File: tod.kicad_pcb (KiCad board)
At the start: 2 copper layers, 72 x 57 mm, 67 parts, among them J1 Conn_01x04, J2 Conn_01x03, J3 Conn_01x04, J4 Conn_01x03, Q1 BC856B, Q2 BC817, Q3 BC856B, Q4 BC817, Q5 BC856, Q6 BC817, Q7 BC856, Q8 BC817, U1 PC817, U2 PC817, U3 PC817, U4 PC817

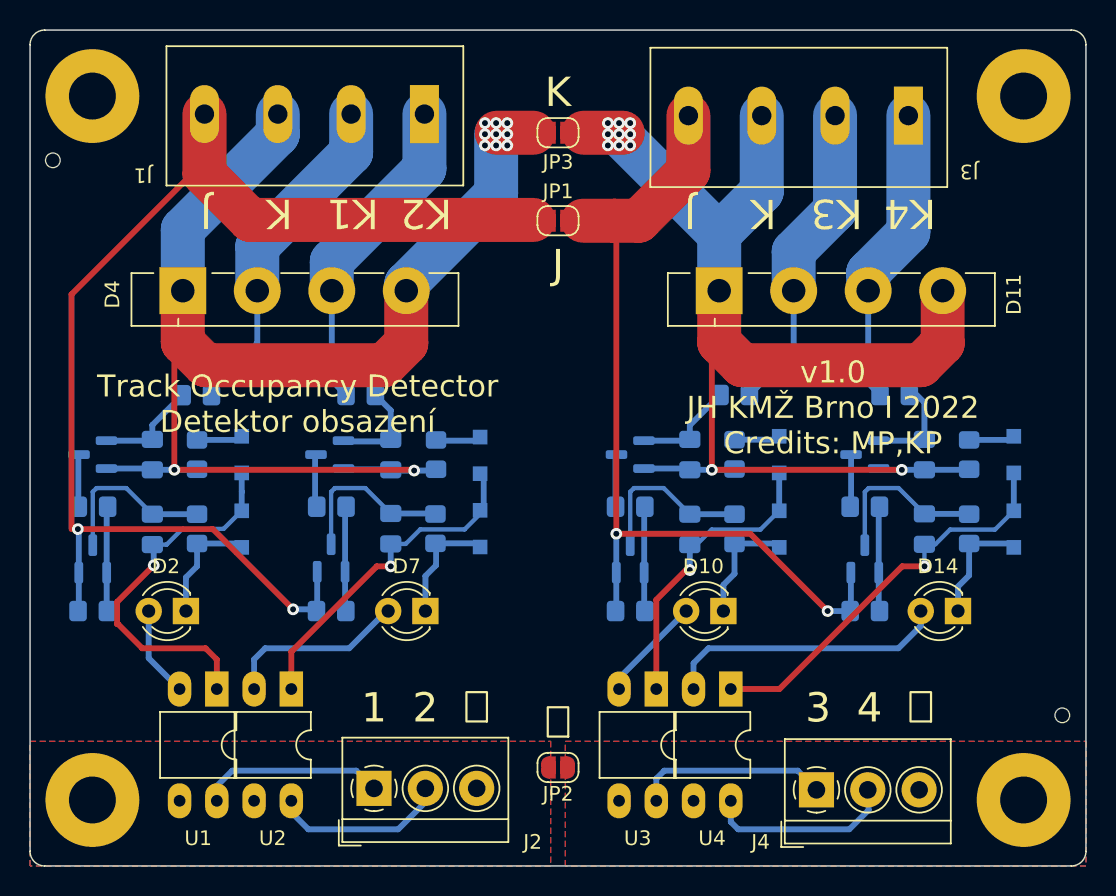
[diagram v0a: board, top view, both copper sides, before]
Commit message: Minor silkscreen tweaks.
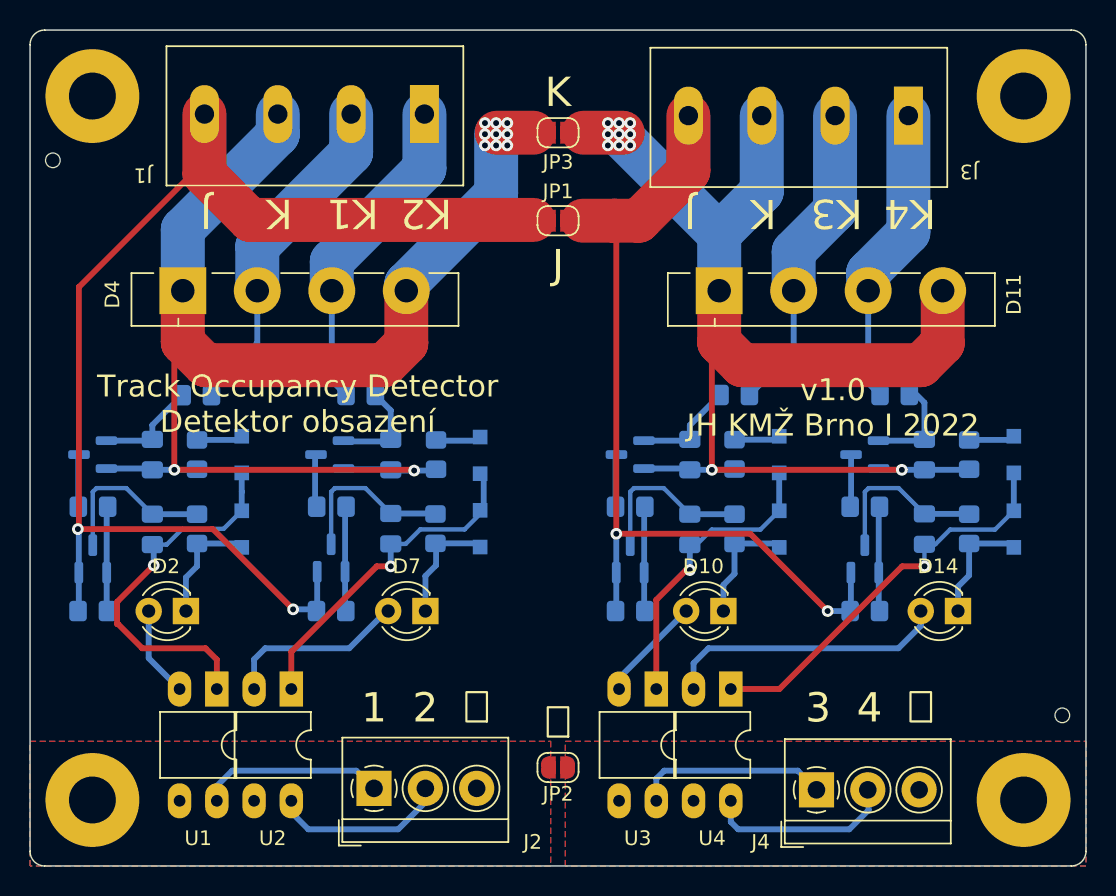
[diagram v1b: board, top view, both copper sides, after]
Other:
- board text added: "v1.0 JH KMŽ Brno I 2022"
- board text removed: "v1.0 JH KMŽ Brno I 2022 Credits: MP,KP"
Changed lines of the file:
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@@
     (effects (font (size 2 2) (thickness 0.15)))
   )
-  (gr_text "v1.0\nJH KMŽ Brno I 2022\nCredits: MP,KP" (at 167.75 88.75) (layer "F.SilkS")
+  (gr_text "v1.0\nJH KMŽ Brno I 2022" (at 167.75 88.75) (layer "F.SilkS")
     (effects (font (size 1.5 1.5) (thickness 0.15)))
   )
@@
   (segment (start 172.212 105.156) (end 159.258 105.156) (width 0.4) (layer "B.Cu") (net 30))
   (segment (start 173.736 102.616) (end 173.736 103.632) (width 0.4) (layer "B.Cu") (net 30))
-  (segment (start 123.824 73.026) (end 123.824 69) (width 0.4) (layer "F.Cu") (net 31))
+  (segment (start 116.332 80.518) (end 116.332 96.954) (width 0.4) (layer "F.Cu") (net 31))
   (segment (start 125.462 97.028) (end 130.934 102.5) (width 0.4) (layer "F.Cu") (net 31))
-  (segment (start 115.824 97.028) (end 115.824 81.026) (width 0.4) (layer "F.Cu") (net 31))
+  (segment (start 116.332 96.954) (end 116.258 97.028) (width 0.4) (layer "F.Cu") (net 31))
   (segment (start 128.016 75.946) (end 147.32 75.946) (width 3) (layer "F.Cu") (net 31))
   (segment (start 124.892 72.822) (end 124.892 68.728) (width 3) (layer "F.Cu") (net 31))
+  (segment (start 123.824 73.026) (end 116.332 80.518) (width 0.4) (layer "F.Cu") (net 31))
   (segment (start 128.016 75.946) (end 124.892 72.822) (width 3) (layer "F.Cu") (net 31))
-  (segment (start 115.824 81.026) (end 123.824 73.026) (width 0.4) (layer "F.Cu") (net 31))
+  (segment (start 123.824 69) (end 123.824 73.026) (width 0.4) (layer "F.Cu") (net 31))
   (segment (start 116.258 97.028) (end 125.462 97.028) (width 0.4) (layer "F.Cu") (net 31))
   (via (at 116.258 97.028) (size 0.8) (drill 0.4) (layers "F.Cu" "B.Cu") (net 31))
